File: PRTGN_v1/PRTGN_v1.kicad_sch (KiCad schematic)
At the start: 1 part

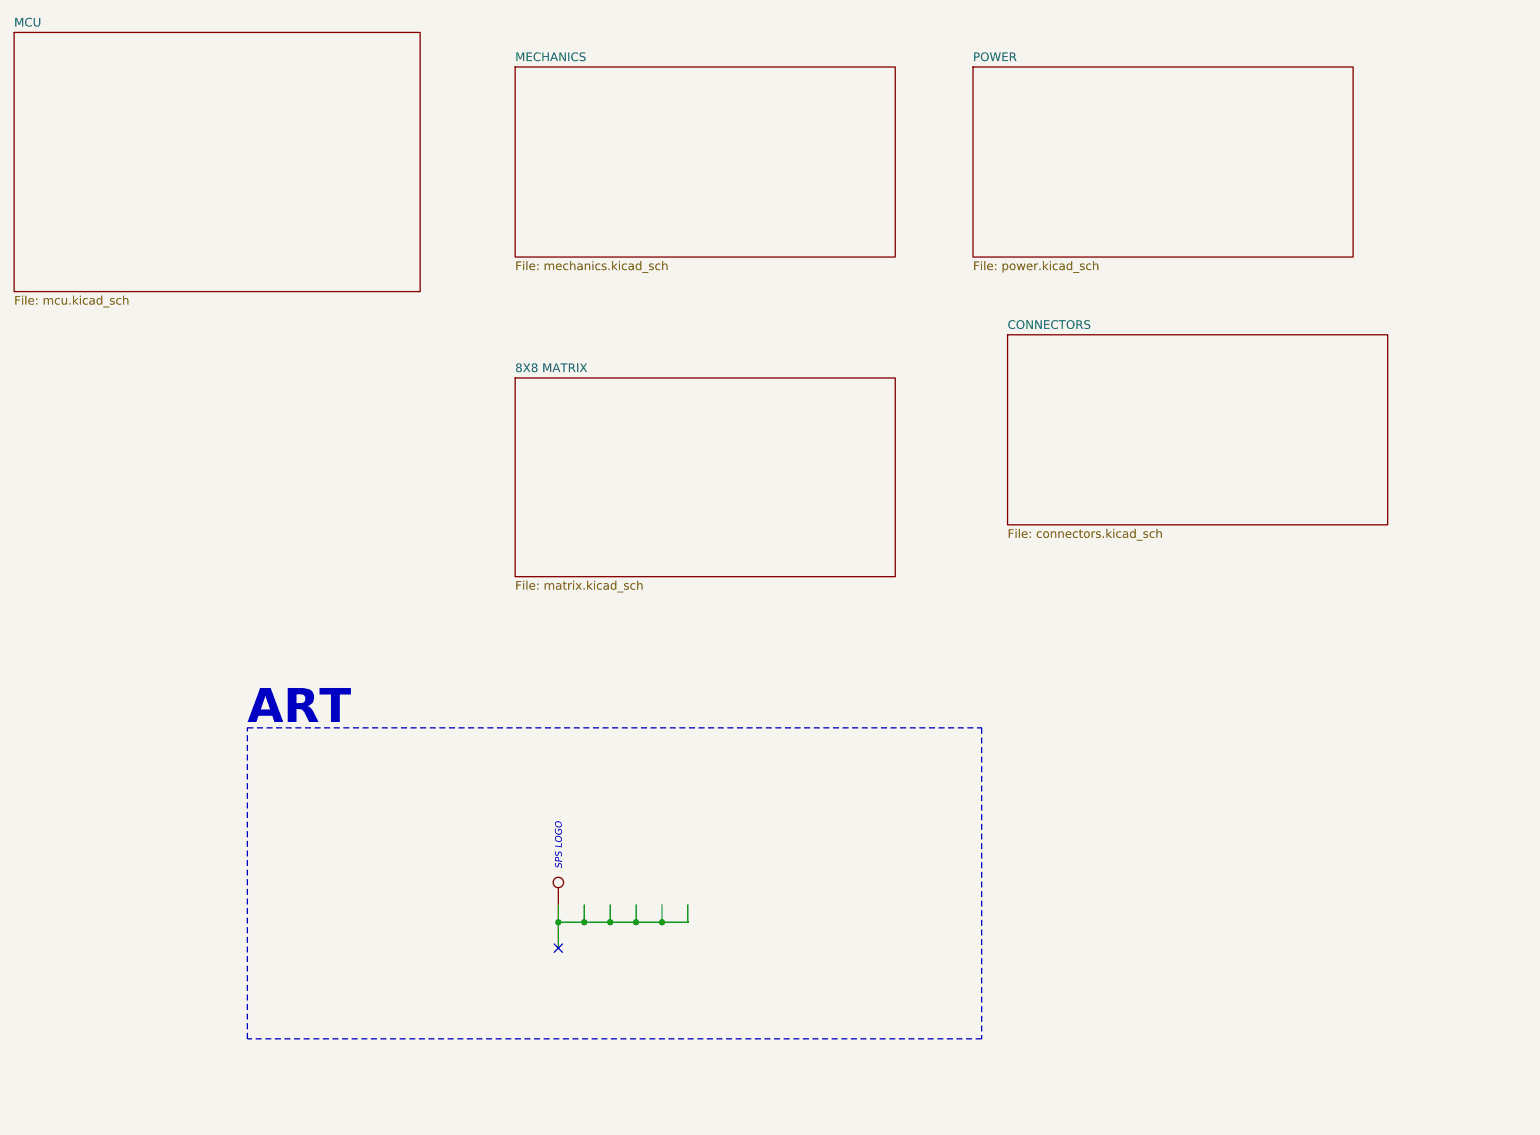
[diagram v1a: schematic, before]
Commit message: PCV updates
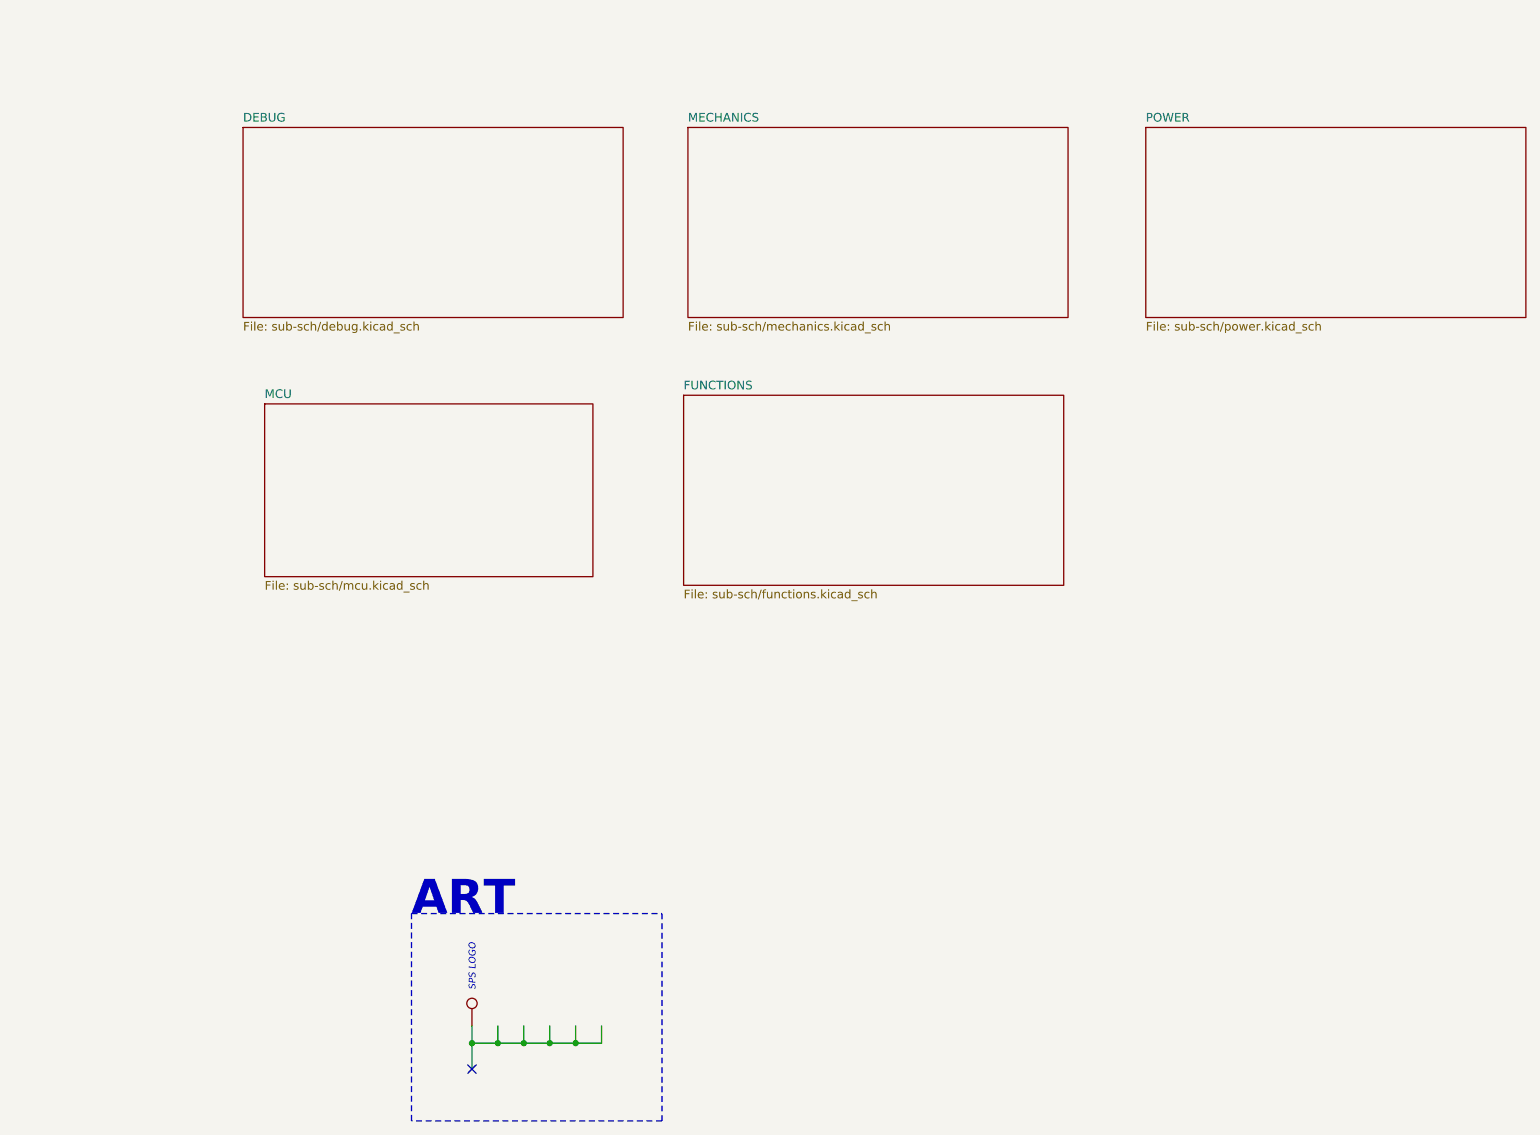
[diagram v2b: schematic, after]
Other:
- sheet CONNECTORS renamed FUNCTIONS
- removed sheet 8X8 MATRIX
- added sheet DEBUG (sub-sch/debug.kicad_sch)
- sheet FUNCTIONS: file connectors.kicad_sch -> sub-sch/functions.kicad_sch
- sheet MCU: file mcu.kicad_sch -> sub-sch/mcu.kicad_sch
- sheet MECHANICS: file mechanics.kicad_sch -> sub-sch/mechanics.kicad_sch
- sheet POWER: file power.kicad_sch -> sub-sch/power.kicad_sch
